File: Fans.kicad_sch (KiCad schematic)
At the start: 4 parts

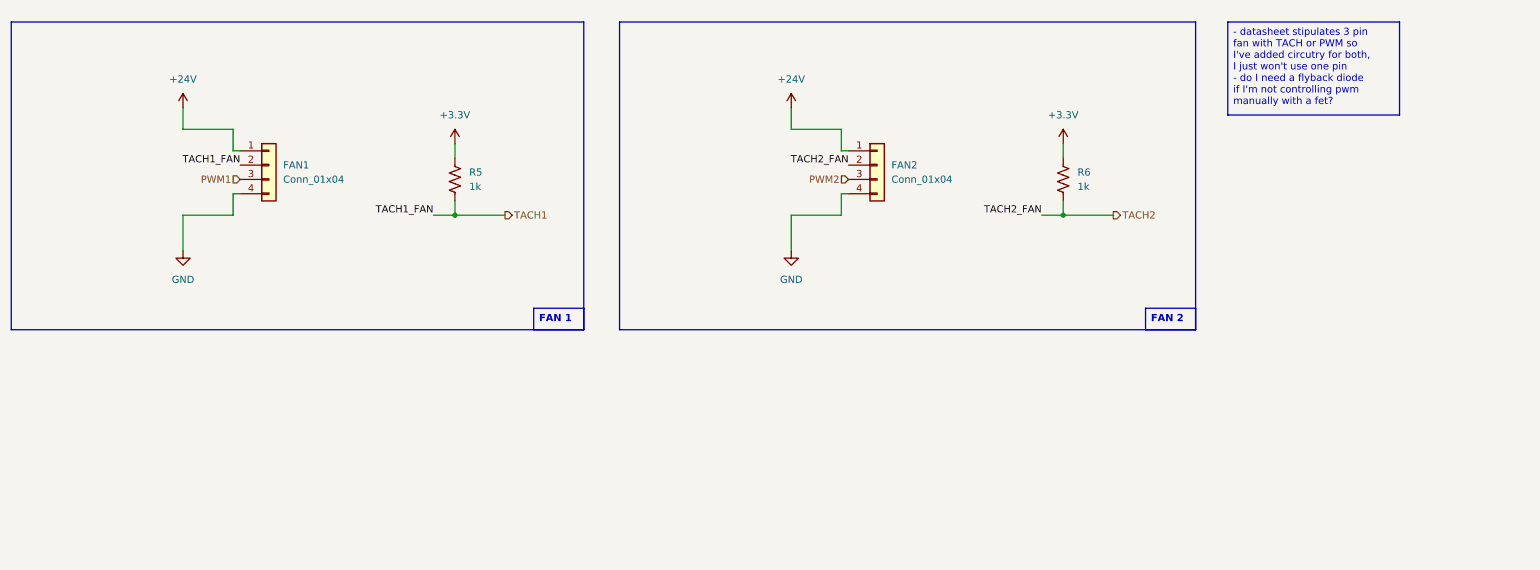
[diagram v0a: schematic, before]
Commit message: added test points and headers, AGND and 12V not fully connected
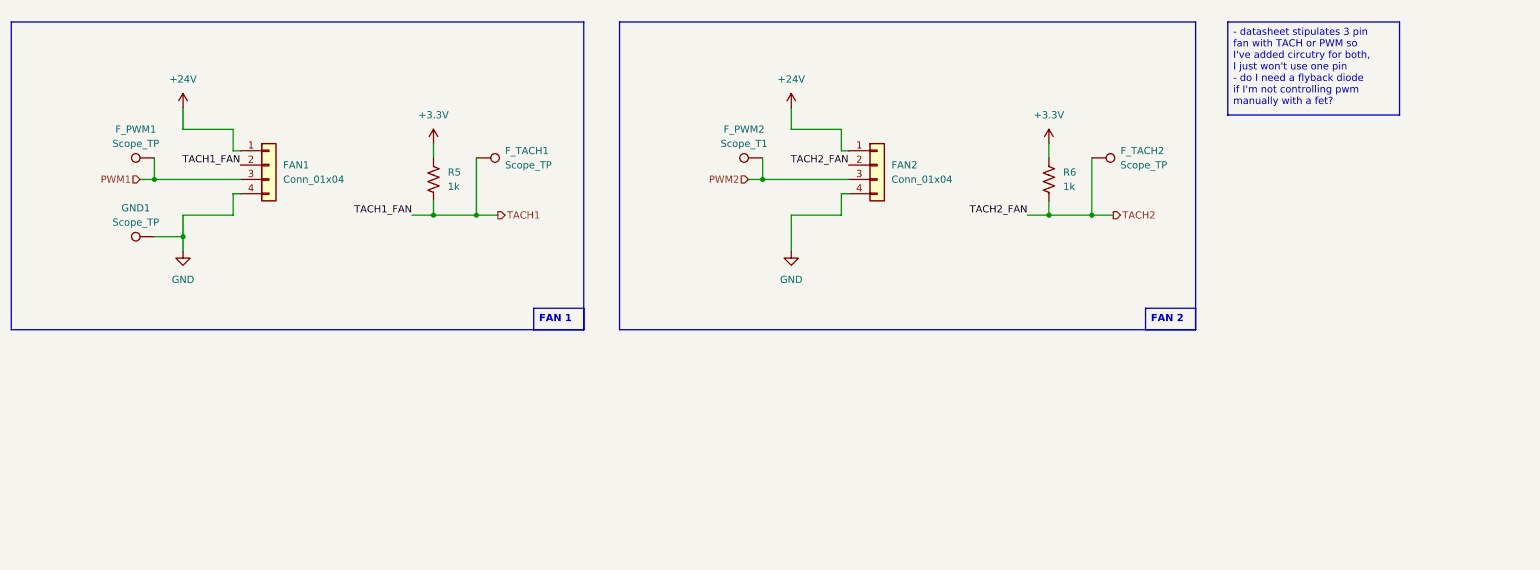
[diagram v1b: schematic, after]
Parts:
- added F_PWM1, F_TACH1, F_TACH2, GND1: Scope_TP, TestPoint:TestPoint_Keystone_5010-5014_Multipurpose, symbol Connector:TestPoint
- added F_PWM2: Scope_T1, TestPoint:TestPoint_Keystone_5010-5014_Multipurpose, symbol Connector:TestPoint
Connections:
- net GND: now also GND1.1
- net PWM1: now also F_PWM1.1
- net PWM2: now also F_PWM2.1
- net TACH1: now also F_TACH1.1
- net TACH2: now also F_TACH2.1
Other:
- moved on the sheet: R5, R6

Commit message: Fixed fan schematic based on review feedback
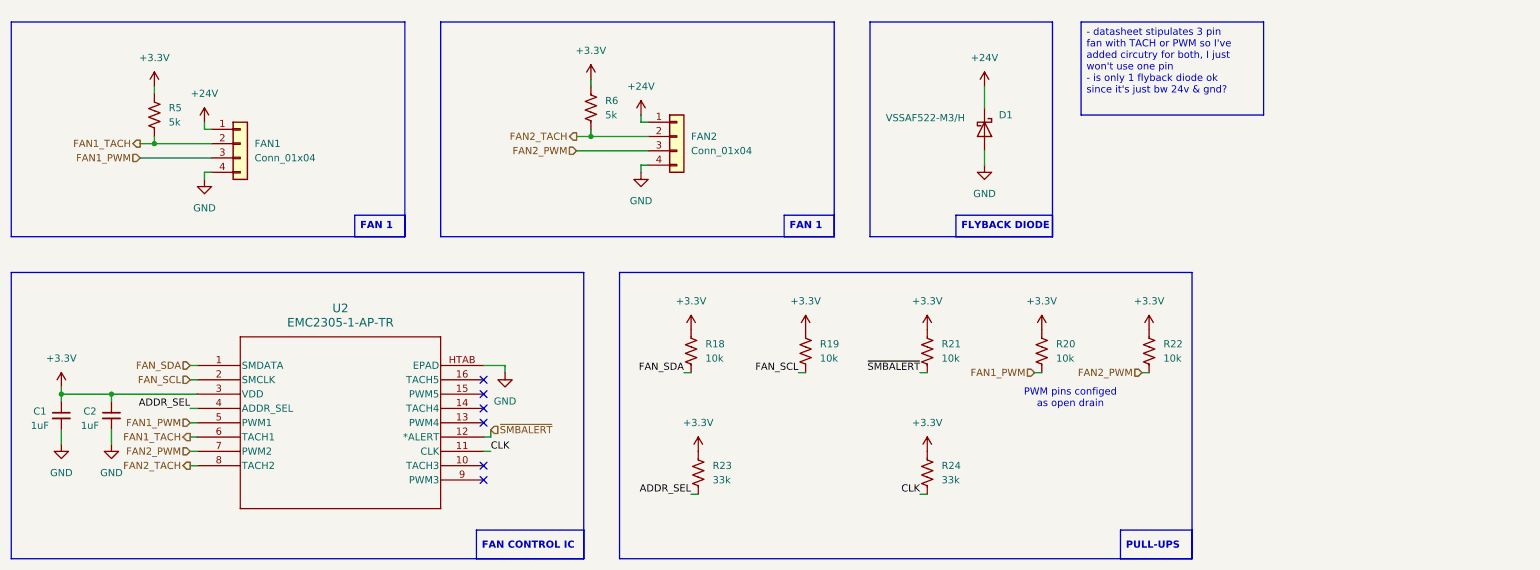
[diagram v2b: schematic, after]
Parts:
- removed F_PWM1, F_TACH1, F_TACH2, GND1: Scope_TP, TestPoint:TestPoint_Keystone_5010-5014_Multipurpose, symbol Connector:TestPoint
- removed F_PWM2: Scope_T1, TestPoint:TestPoint_Keystone_5010-5014_Multipurpose, symbol Connector:TestPoint
- added C1, C2: 1uF, Capacitor_SMD:C_0805_2012Metric, symbol Device:C_Small
- added D1: VSSAF522-M3/H, UTSVT_Passive:DO-221AC, symbol Diode:C3D25170H
- added R18, R19, R20, R21, R22: 10k, Resistor_SMD:R_0805_2012Metric, symbol Device:R_US
- added R23, R24: 33k, Resistor_SMD:R_0805_2012Metric, symbol Device:R_US
- added U2: EMC2305-1-AP-TR, FanControl:QFN16_4x4MC_MCH, symbol 2024-11-02_21-04-42:EMC2305-1-AP-TR
- FAN1, FAN2: Notes Small signal control for pump -> (none)
- R5, R6: value 1k -> 5k
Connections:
- net +24V: now also D1.1 (K)
- net +3.3V: now also C1.1, C2.1, R18.2, R19.2, R20.2, R21.2, R22.2, R23.2, R24.2, U2.3 (VDD)
- net GND: now also C1.2, C2.2, D1.2 (A), U2.HTAB (EPAD)
- net PWM1 renamed FAN1_PWM
- net FAN1_PWM: now also R20.1, U2.5 (PWM1)
- net PWM2 renamed FAN2_PWM
- net FAN2_PWM: now also R22.1, U2.7 (PWM2)
- net TACH1 renamed FAN1_TACH
- net FAN1_TACH: now also U2.6 (TACH1)
- net TACH2 renamed FAN2_TACH
- net FAN2_TACH: now also U2.8 (TACH2)
- new net ADDR_SEL: R23.1, U2.4 (ADDR_SEL)
- new net CLK: R24.1, U2.11 (CLK)
- new net FAN_SCL: R19.1, U2.2 (SMCLK)
- new net FAN_SDA: R18.1, U2.1 (SMDATA)
- new net ~{SMBALERT}: R21.1, U2.12 (*ALERT)
- no-connect marks 0 -> 6
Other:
- note added: "PWM pins configed as open drain"
- moved on the sheet: FAN1, FAN2, R5, R6

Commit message: updated schematic with low pass for temp sensors and new resistor footprint
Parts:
- R18, R19, R20, R21, R22, R23, R24, R5, R6: footprint Resistor_SMD:R_0805_2012Metric -> Resistor_SMD:R_0603_1608Metric

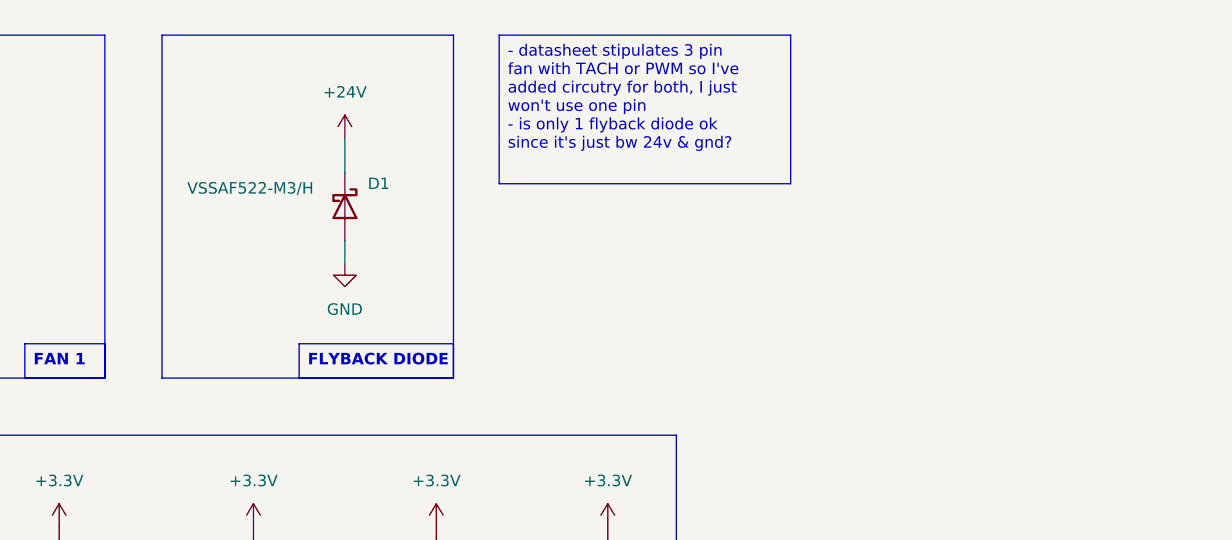
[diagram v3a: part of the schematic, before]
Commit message: low pass for temp & flyback diodes
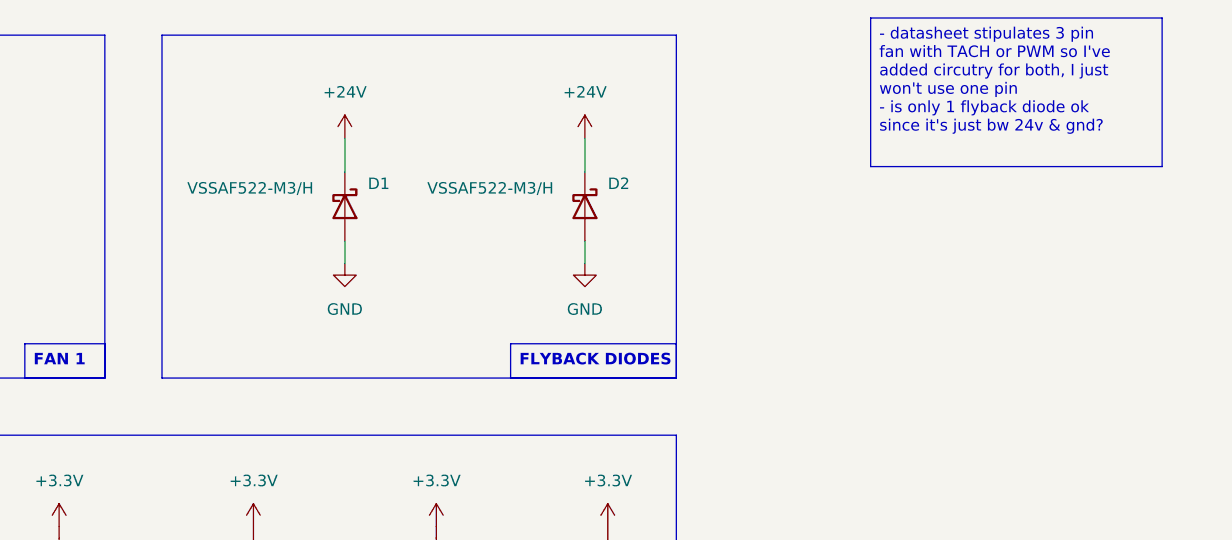
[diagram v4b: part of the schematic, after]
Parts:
- added D2: VSSAF522-M3/H, UTSVT_Passive:DO-221AC, symbol Diode:C3D25170H
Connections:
- net +24V: now also D2.1 (K)
- net GND: now also D2.2 (A)
